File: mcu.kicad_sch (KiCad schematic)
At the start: 44 parts, among them J1 SWD_3.3V, J2 Connector, USB-TYPE-C-16P, J3 SWD_GND, J4 SWD_SWDIO, J5 SWD_SWCLK, U1 SN74AHCT1G125DBVR, U2 STM32F723VET6, U3 TS3USB221ARSER, U4 USBLC6-2SC6, X1 16MHz

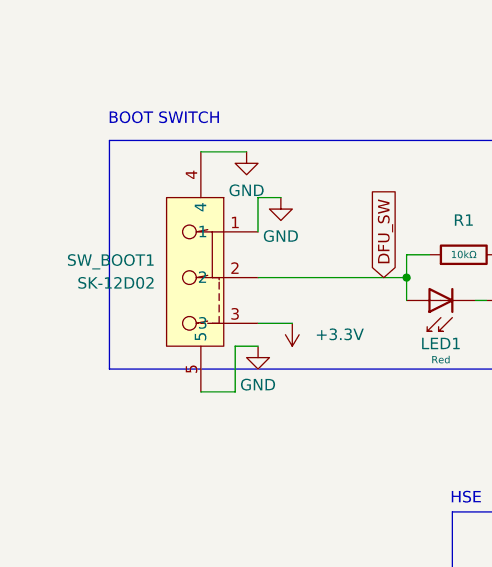
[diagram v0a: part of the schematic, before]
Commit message: lcsc part
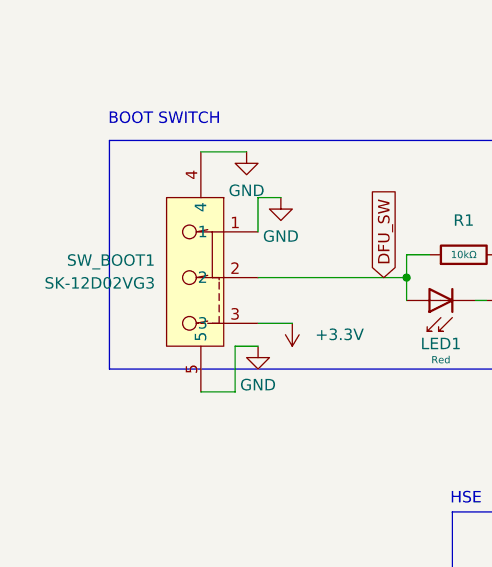
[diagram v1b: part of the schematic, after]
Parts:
- F1: LCSC (none) -> C1512049
- J1, J3, J4, J5: now left out of the parts list
- RV1: LCSC (none) -> C470754
- SW_BOOT1: value SK-12D02 -> SK-12D02VG3; LCSC (none) -> C131374
- U2: LCSC (none) -> C5270022
- U3: LCSC (none) -> C128396
- U4: LCSC (none) -> C7519
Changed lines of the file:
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@@
 			)
 		)
-		(property "Value" "SK-12D02"
+		(property "Value" "SK-12D02VG3"
 			(at 31.75 85.7249 90)
 			(show_name no)
@@
 			)
 		)
+		(property "LCSC" "C131374"
+			(at 39.37 83.82 90)
+			(hide yes)
+			(show_name no)
+			(do_not_autoplace no)
+			(effects
+				(font
+					(size 1.27 1.27)
+				)
+			)
+		)
 		(pin "2"
 		)
@@
 			)
 		)
+		(property "LCSC" "C7519"
+			(at 330.2 190.5 0)
+			(hide yes)
+			(show_name no)
+			(do_not_autoplace no)
+			(effects
+				(font
+					(size 1.27 1.27)
+				)
+			)
+		)
 		(pin "1"
 		)
@@
 			)
 		)
+		(property "LCSC" "C1512049"
+			(at 353.06 233.68 0)
+			(hide yes)
+			(show_name no)
+			(do_not_autoplace no)
+			(effects
+				(font
+					(size 1.27 1.27)
+				)
+			)
+		)
 		(pin "1"
 		)
@@
 		(body_style 1)
 		(exclude_from_sim no)
-		(in_bom yes)
+		(in_bom no)
 		(on_board yes)
 		(in_pos_files yes)
@@
 		(body_style 1)
 		(exclude_from_sim no)
-		(in_bom yes)
+		(in_bom no)
 		(on_board yes)
 		(in_pos_files yes)
@@
 			)
 		)
+		(property "LCSC" "C128396"
+			(at 238.76 182.88 0)
+			(hide yes)
+			(show_name no)
+			(do_not_autoplace no)
+			(effects
+				(font
+					(size 1.27 1.27)
+				)
+			)
+		)
 		(pin "3"
 		)
@@
 			)
 		)
+		(property "LCSC" "C5270022"
+			(at 162.56 149.86 0)
+			(hide yes)
+			(show_name no)
+			(do_not_autoplace no)
+			(effects
+				(font
+					(size 1.27 1.27)
+				)
+			)
+		)
 		(pin "13"
 		)
@@
 		(body_style 1)
 		(exclude_from_sim no)
-		(in_bom yes)
+		(in_bom no)
 		(on_board yes)
 		(in_pos_files yes)
@@
 		(body_style 1)
 		(exclude_from_sim no)
-		(in_bom yes)
+		(in_bom no)
 		(on_board yes)
 		(in_pos_files yes)
@@
 			)
 		)
+		(property "LCSC" "C470754"
+			(at 275.59 111.76 0)
+			(hide yes)
+			(show_name no)
+			(do_not_autoplace no)
+			(effects
+				(font
+					(size 1.27 1.27)
+				)
+			)
+		)

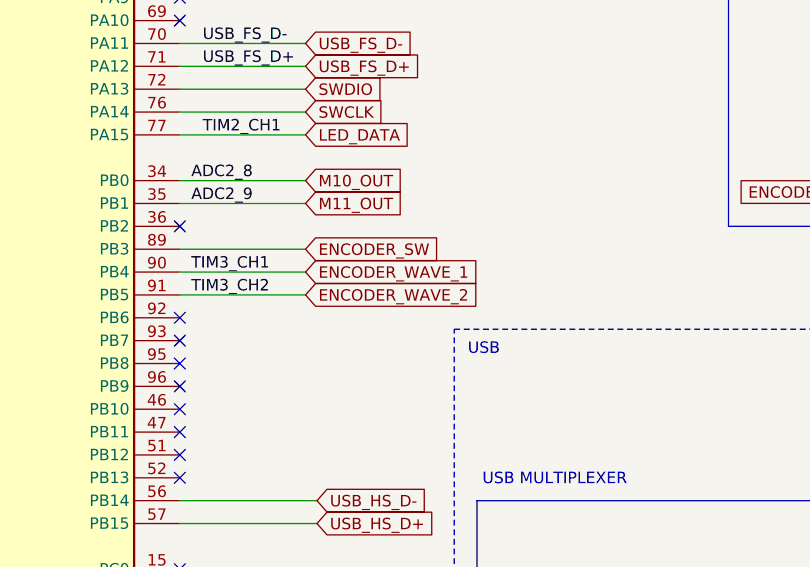
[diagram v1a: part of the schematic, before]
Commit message: fix
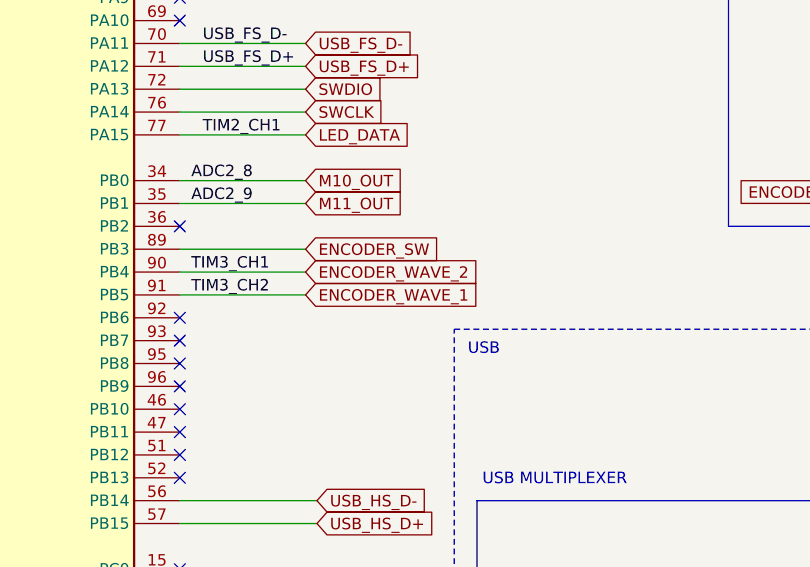
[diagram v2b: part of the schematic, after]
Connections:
- net ENCODER_WAVE_1: now also U2.91 (PB5); no longer U2.90 (PB4)
- net ENCODER_WAVE_2: now also U2.90 (PB4); no longer U2.91 (PB5)
